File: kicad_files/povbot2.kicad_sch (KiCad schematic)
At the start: 22 parts, among them J1 GPIO, J2 TYPE-C-31-M-12, U1 TPS61232DRC, U2 DRV8837, U3 DRV8837, U4 MCP73831-2ACI_MC, U5 AP2112K-3.3

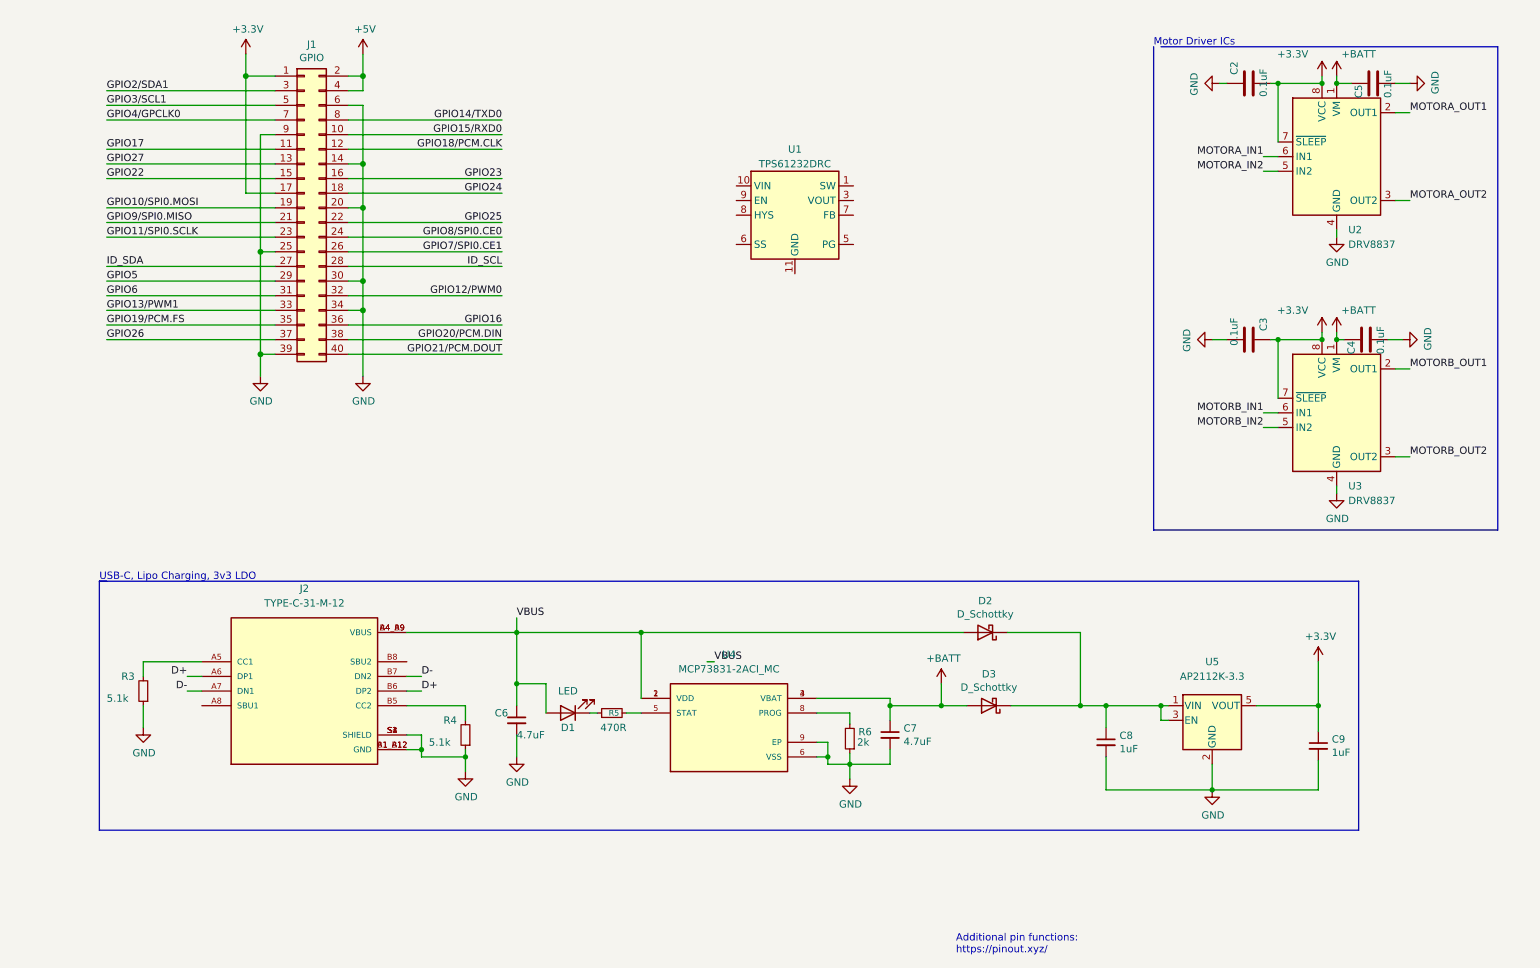
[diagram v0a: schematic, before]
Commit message: added motor driver IC, BOM, laser diode, LEDs, and electomagnet
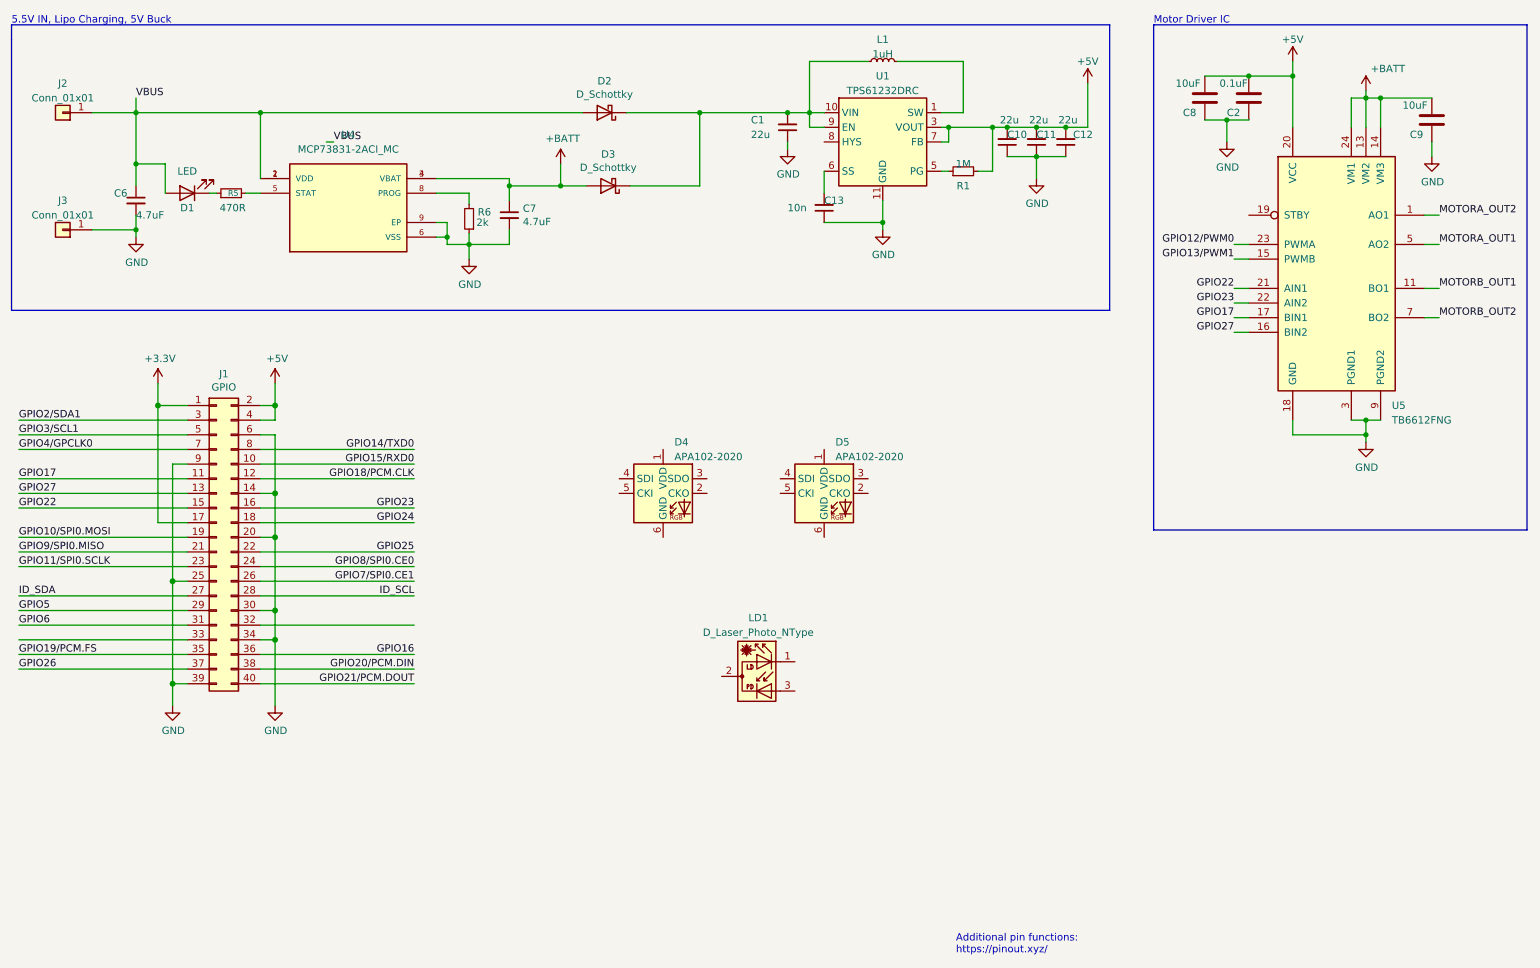
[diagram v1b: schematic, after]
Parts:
- removed C3, C4, C5: 0.1uF, Capacitor_SMD:C_0402_1005Metric, symbol Device:C
- removed C8, C9: 1uF, Capacitor_SMD:C_0402_1005Metric, symbol Device:C_Small
- removed J2: TYPE-C-31-M-12, kicad_footprints:HRO_TYPE-C-31-M-12, symbol Kicad_symbols:TYPE-C-31-M-12
- removed R3, R4: 5.1k, Resistor_SMD:R_0402_1005Metric, symbol Device:R_Small
- removed U2, U3: DRV8837, Package_SON:WSON-8-1EP_2x2mm_P0.5mm_EP0.9x1.6mm, symbol Driver_Motor:DRV8837
- removed U5: AP2112K-3.3, Package_TO_SOT_SMD:SOT-23-5, symbol Regulator_Linear:AP2112K-3.3
- added C1, C10, C11, C12: 22u, symbol Device:C_Small
- added C13: 10n, symbol Device:C_Small
- added C8, C9: 10uF, Capacitor_SMD:C_0402_1005Metric, symbol Device:C
- added D4, D5: APA102-2020, LED_SMD:LED-APA102-2020, symbol LED:APA102-2020
- added J2, J3: Conn_01x01, symbol Connector_Generic:Conn_01x01
- added L1: 1uH, symbol Device:L_Small
- added LD1: D_Laser_Photo_NType, symbol Device:D_Laser_Photo_NType
- added R1: 1M, symbol Device:R_Small
- added U5: TB6612FNG, Package_SO:SSOP-24_5.3x8.2mm_P0.65mm, symbol Driver_Motor:TB6612FNG
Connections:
- net +3V3: no longer C2.1
- net +5V: now also C2.1, U1.3 (VOUT), U1.4 (VOUT), U1.7 (FB), C10.2, C11.2, C12.2, C8.1, R1.2, U5.20 (VCC)
- net +BATT: now also C9.1, U5.13 (VM2), U5.14 (VM3), U5.24 (VM1)
- net GND: now also U1.11 (GND), C1.1, C10.1, C11.1, C12.1, C13.1, C8.2, C9.2, J3.1 (Pin_1), U5.10 (PGND2), U5.18 (GND), U5.3 (PGND1), U5.4 (PGND1), U5.9 (PGND2)
- net GPIO12/PWM0: now also U5.23 (PWMA); no longer J1.32 (Pin_32)
- net GPIO13/PWM1: now also U5.15 (PWMB); no longer J1.33 (Pin_33)
- net GPIO17: now also U5.17 (BIN1)
- net GPIO22: now also U5.21 (AIN1)
- net GPIO23: now also U5.22 (AIN2)
- net GPIO27: now also U5.16 (BIN2)
- net MOTORA_OUT1: now also U5.5 (AO2), U5.6 (AO2)
- net MOTORA_OUT2: now also U5.1 (AO1), U5.2 (AO1)
- net MOTORB_OUT1: now also U5.11 (BO1), U5.12 (BO1)
- net MOTORB_OUT2: now also U5.7 (BO2), U5.8 (BO2)
- net VBUS: now also J2.1 (Pin_1)
- net at D2.1 (K), D3.1 (K): now also U1.10 (VIN), U1.9 (EN), C1.2, L1.1
- net at U1.1 (SW), U1.2 (SW): now also L1.2
- net at U1.5 (PG): now also R1.1
- net at U1.6 (SS): now also C13.2
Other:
- note added: "5.5V IN, Lipo Charging, 5V Buck"
- note added: "Motor Driver IC"
- note removed: "Motor Driver ICs"
- note removed: "USB-C, Lipo Charging, 3v3 LDO"
- moved on the sheet: C2, C6, C7, D1, D2, D3, J1, R5, R6, U1, U4
